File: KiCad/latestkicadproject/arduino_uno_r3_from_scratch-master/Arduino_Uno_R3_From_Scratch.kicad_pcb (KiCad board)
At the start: 2 copper layers, 50.8 x 58.4 mm, 36 parts, among them IC1 MC33269ST-5.OT3, IC2 MC33269ST-5.OT3, IC3 L298P, IC5 ATMEGA328P-MU, P1 CONN_01X06, P2 IOH, P3 AD, P4 H4, SW1 RESET_SWITCH, U3 74AHC1G04, U4 74AHC1G04, X1 DG3XX-04-3.5, X2 DG3XX-02-3.5, Y2 Crystal

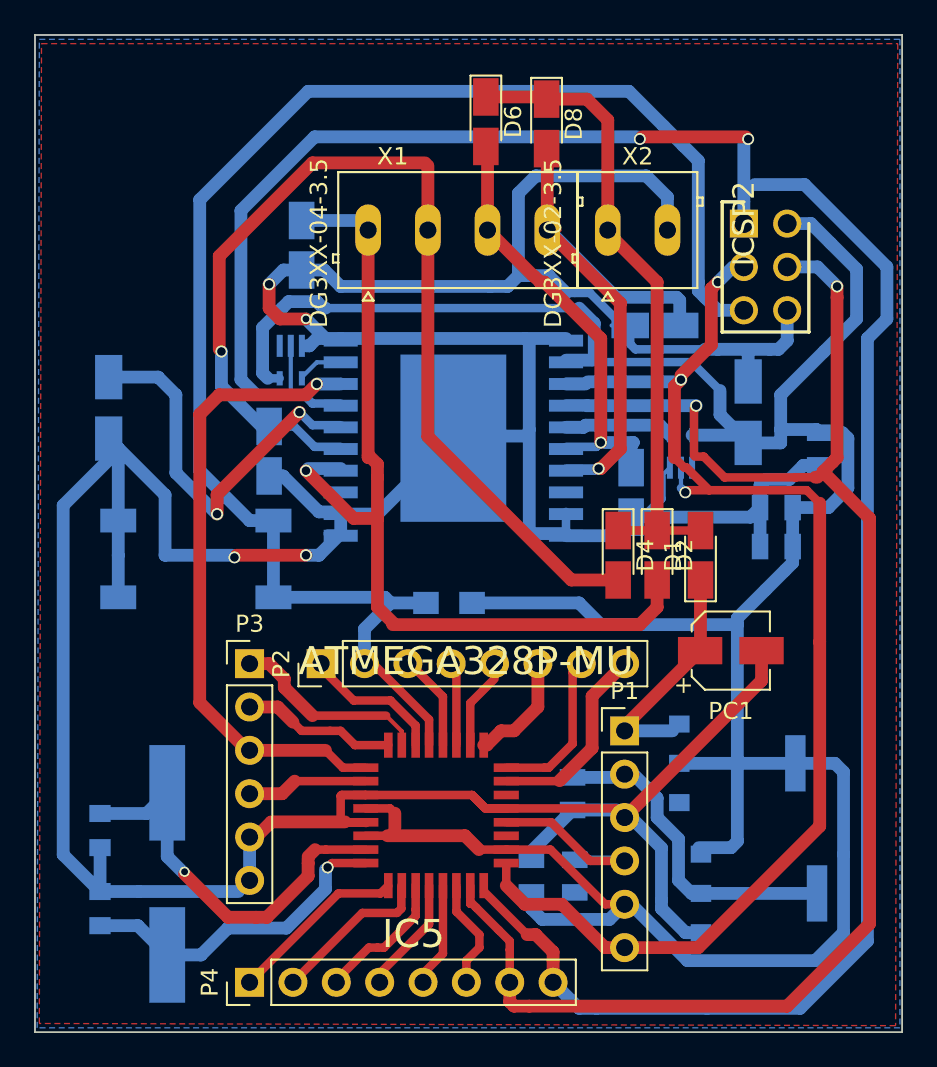
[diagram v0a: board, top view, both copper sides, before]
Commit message: verbeteringen kicad
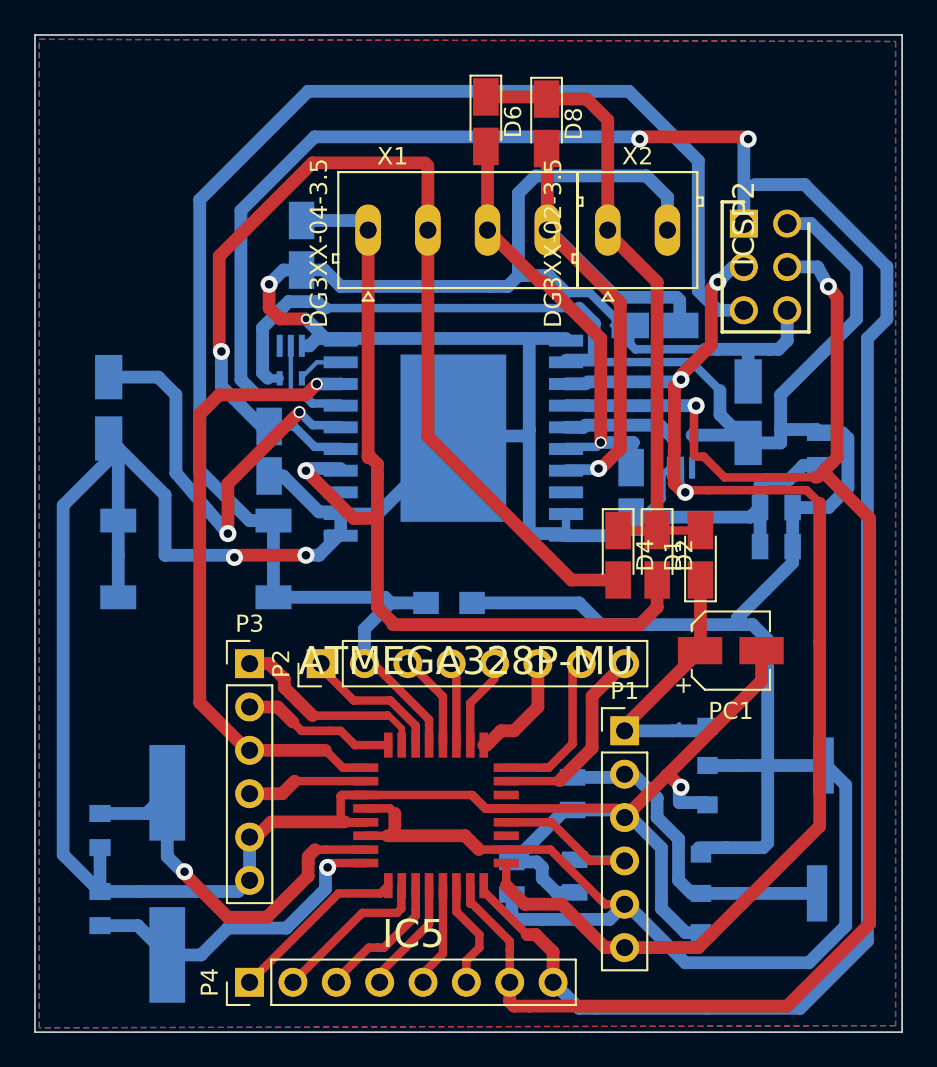
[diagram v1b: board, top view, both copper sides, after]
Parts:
- moved IC1 1.66 mm to (101.0, 98.3)
- moved C6 1.15 mm to (86.1, 104.9)
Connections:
- C4 pad 2: Net-(C4-Pad2) -> GND
- IC1 pad 1: Net-(IC1-Pad1) -> GND
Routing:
- net GND: track 301.7 -> 304.3 mm, vias 4 -> 5
- net +5V: track 186.3 -> 188.7 mm
- net /Headers/VIN: track 14.2 -> 16.3 mm
- net /Driver/PWRIN: track 23.1 -> 25.2 mm
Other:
- net class 15mills added: clearance 0.25, trace_width 0.38, via_dia 0.6, via_drill 0.4
- net class 30mills: via_dia 0.7 -> 1
